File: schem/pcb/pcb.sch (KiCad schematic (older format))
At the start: 8 parts, among them J101 2x3 female, J102 2x3 female, U101 74HCT245, U102 BP, U103 74HC165, U104 74HC595

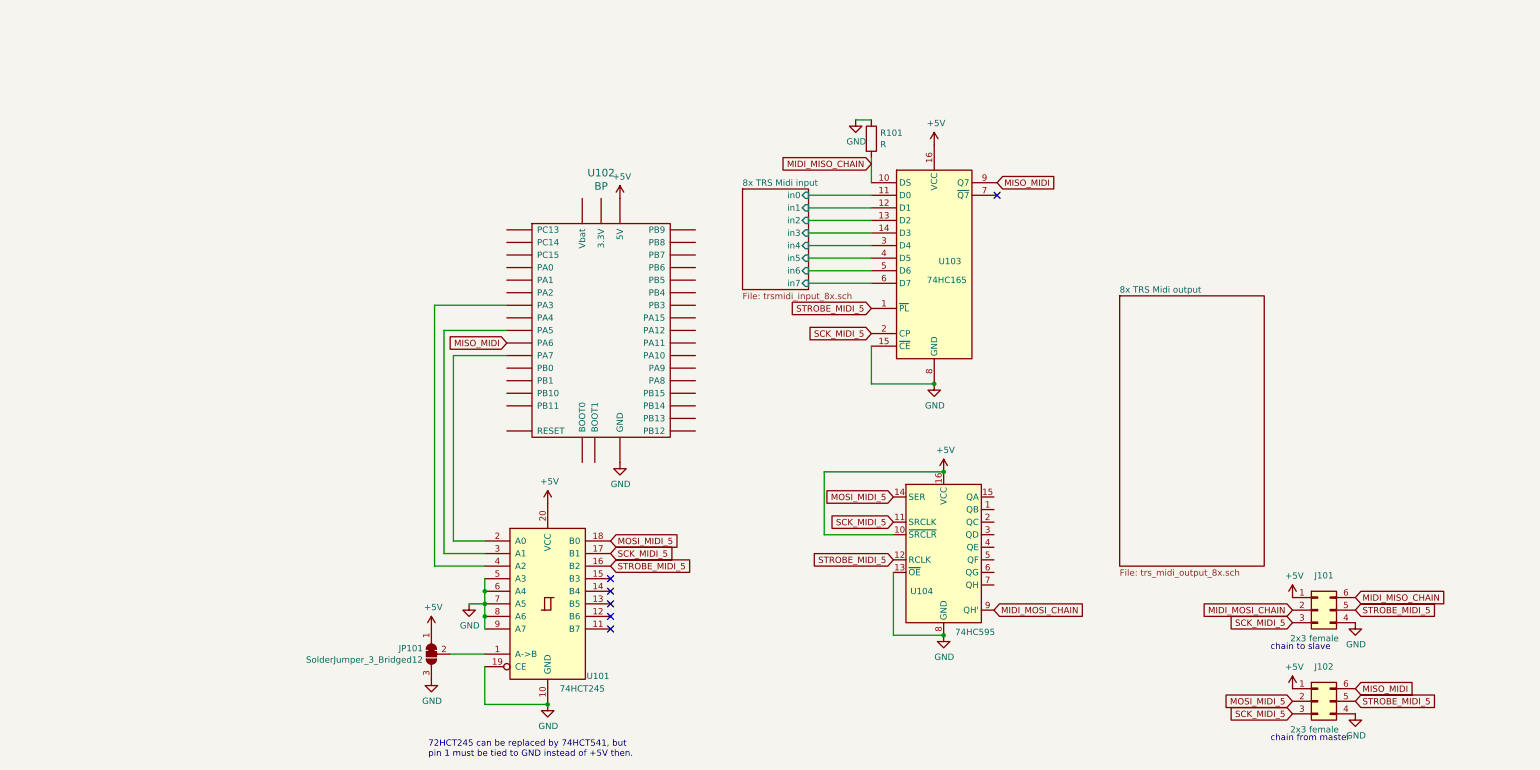
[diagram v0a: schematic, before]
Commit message: First attempts at a PCB layout...
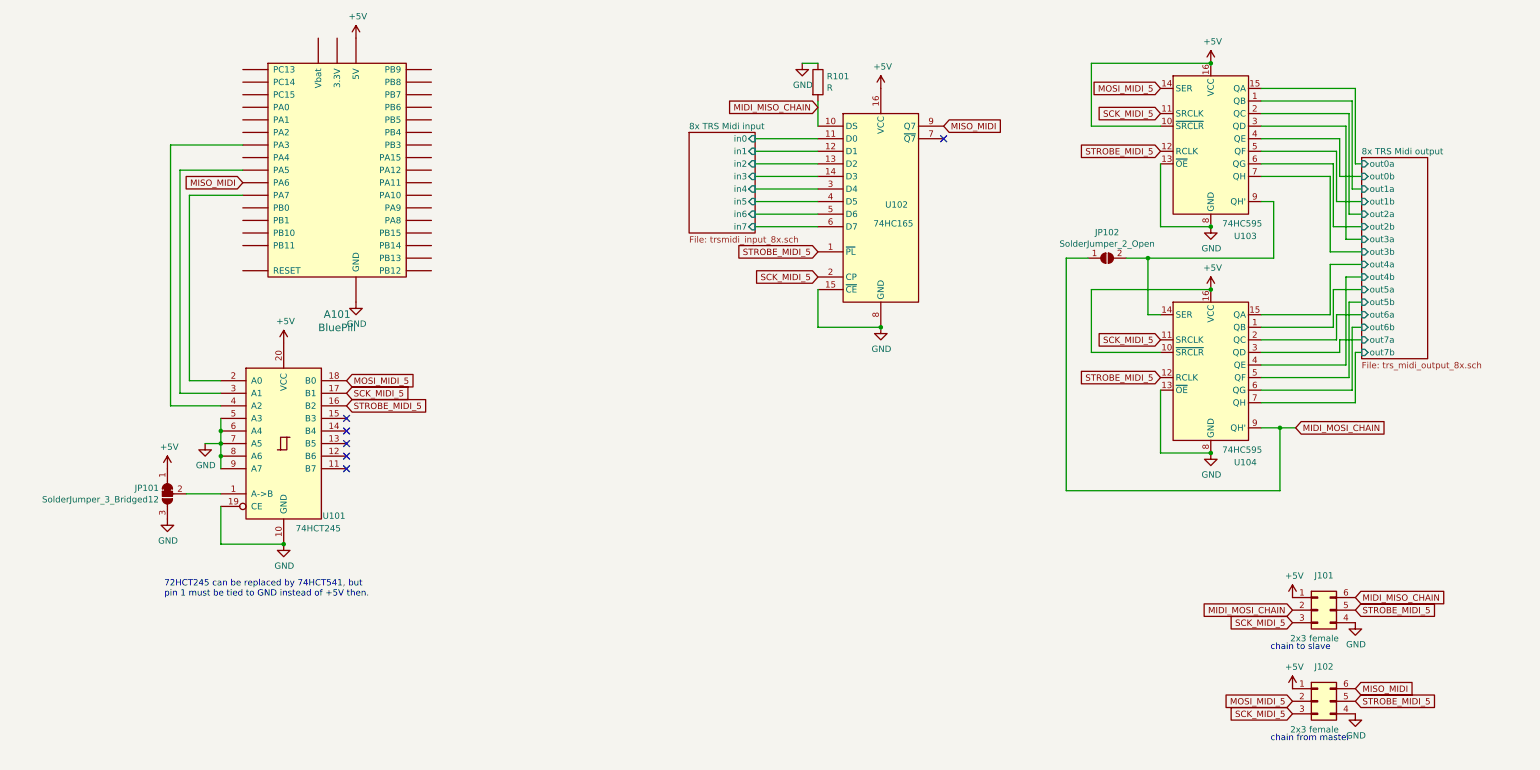
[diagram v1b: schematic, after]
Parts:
- removed U102: BP, symbol bluepill:BP
- added A101: BluePill, footprints:BLUEPILL, symbol bluepill:BluePill
- added JP102: SolderJumper_2_Open, Jumper:SolderJumper-2_P1.3mm_Open_TrianglePad1.0x1.5mm, symbol Jumper:SolderJumper_2_Open
- added U104: 74HC595, Package_DIP:DIP-16_W7.62mm, symbol 74xx:74HC595
- J101, J102: footprint (none) -> Connector_PinHeader_2.54mm:PinHeader_2x03_P2.54mm_Vertical
- JP101: footprint (none) -> Jumper:SolderJumper-3_P2.0mm_Open_TrianglePad1.0x1.5mm
- R101: footprint (none) -> Resistor_SMD:R_0805_2012Metric
- U101: footprint (none) -> Package_DIP:DIP-20_W7.62mm
- U102: renamed from U103; footprint (none) -> Package_DIP:DIP-16_W7.62mm
- U103: renamed from U104; footprint (none) -> Package_DIP:DIP-16_W7.62mm
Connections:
- net +5V: now also A101.5V, U104.10 (~SRCLR), U104.16 (VCC)
- net GND: now also A101.G (GND), U104.13 (~OE), U104.8 (GND)
- net MIDI_MOSI_CHAIN: now also JP102.1 (A), U104.9 (QH'); no longer U103.9 (QH')
- net MISO_MIDI: now also A101.PA6
- net SCK_MIDI_5: now also U104.11 (SRCLK)
- net STROBE_MIDI_5: now also U104.12 (RCLK)
- net 8x TRS Midi output/out1a: now reaches U103.1 (QB)
- net 8x TRS Midi output/out0a: now reaches U103.15 (QA)
- net 8x TRS Midi output/out2a: now reaches U103.2 (QC)
- net 8x TRS Midi output/out3a: now reaches U103.3 (QD)
- net 8x TRS Midi output/out0b: now reaches U103.4 (QE)
- net 8x TRS Midi output/out1b: now reaches U103.5 (QF)
- net 8x TRS Midi output/out2b: now reaches U103.6 (QG)
- net 8x TRS Midi output/out3b: now reaches U103.7 (QH)
- net at U101.4 (A2): now also A101.PA3
- net at U101.3 (A1): now also A101.PA5
- net at U101.2 (A0): now also A101.PA7
- new net: JP102.2 (B), U103.9 (QH'), U104.14 (SER)
- new net 8x TRS Midi output/out4a: U104.15 (QA)
- new net 8x TRS Midi output/out4b: U104.4 (QE)
- new net 8x TRS Midi output/out5a: U104.1 (QB)
- new net 8x TRS Midi output/out5b: U104.5 (QF)
- new net 8x TRS Midi output/out6a: U104.2 (QC)
- new net 8x TRS Midi output/out6b: U104.6 (QG)
- new net 8x TRS Midi output/out7a: U104.3 (QD)
- new net 8x TRS Midi output/out7b: U104.7 (QH)
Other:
- moved on the sheet: JP101, R101, U101, U102, U103
